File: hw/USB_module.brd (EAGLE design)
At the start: 25 x 45 mm, 39 parts, among them J1 GROVE-4P-2.0-3470130P1, J2 GROVE-4P-2.0-3470130P1, J4 MICRO-USB-5P-340015001, X5 53047-04

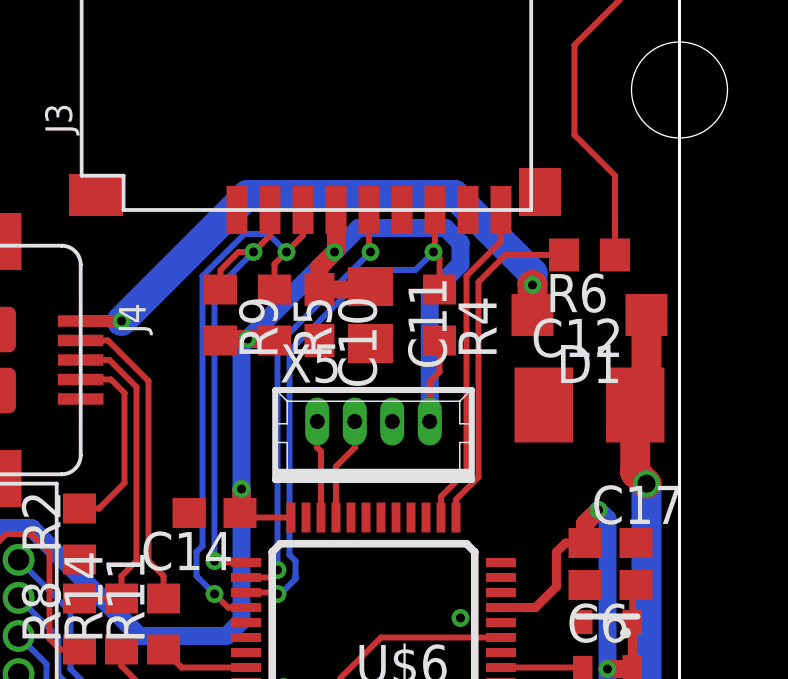
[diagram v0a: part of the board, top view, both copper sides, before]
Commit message: layout completed
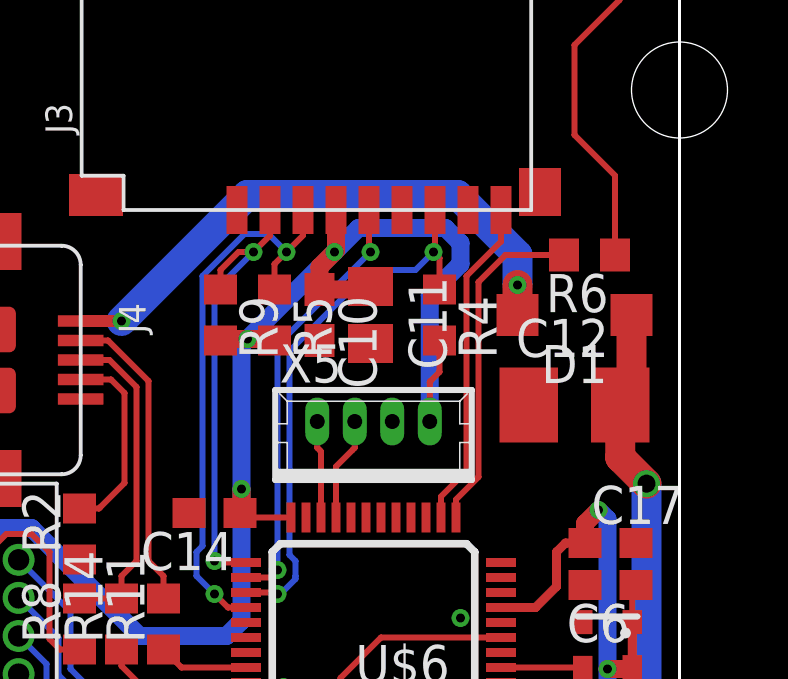
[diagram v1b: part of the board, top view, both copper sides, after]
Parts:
- R4, R5, R9: value 100k -> 47k
- moved C12 0.50 mm to (21.5, 24.5)
- moved D1 0.50 mm to (21.5, 27.5)
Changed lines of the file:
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@@
 <element name="R2" library="rcl" package="R0603" value="100k" x="5" y="20.2" rot="R90"/>
 <element name="R8" library="rcl" package="R0603" value="1k5" x="5" y="17.2" rot="R90"/>
-<element name="D1" library="diode" package="SOD123" value="MBR0520LT" x="22" y="27.5" rot="R180"/>
+<element name="D1" library="diode" package="SOD123" value="MBR0520LT" x="21.5" y="27.5" rot="R180"/>
 <element name="J3" library="OPL-Connector" package="9+4P-SMD-L16.1*W14.5*H1.85MM" value="" x="12.5" y="31" rot="R90"/>
-<element name="R4" library="rcl" package="R0603" value="100k" x="17" y="27.5" rot="R270"/>
-<element name="R5" library="rcl" package="R0603" value="100k" x="11.5" y="27.5" rot="R270"/>
-<element name="R9" library="rcl" package="R0603" value="100k" x="9.7" y="27.5" rot="R270"/>
+<element name="R4" library="rcl" package="R0603" value="47k" x="17" y="27.5" rot="R270"/>
+<element name="R5" library="rcl" package="R0603" value="47k" x="11.5" y="27.5" rot="R270"/>
+<element name="R9" library="rcl" package="R0603" value="47k" x="9.7" y="27.5" rot="R270"/>
 <element name="J4" library="OPL Eagle Library" package="B-SMD-5P" value="MICRO-USB-5P-340015001" x="2.5" y="26" rot="R270"/>
 <element name="C10" library="rcl" package="C0603" value="100n" x="13" y="27.5" rot="R270"/>
 <element name="C11" library="rcl" package="C0805" value="4.7u" x="14.7" y="27.5" rot="R270"/>
-<element name="C12" library="rcl" package="B/3528-21R" value="" x="22" y="24.5"/>
+<element name="C12" library="rcl" package="B/3528-21R" value="" x="21.5" y="24.5"/>
 <element name="LED2" library="led" package="CHIPLED_0805" value="" x="23" y="42.5" rot="R180"/>
 <element name="R6" library="rcl" package="R0603" value="330" x="22" y="29.5" rot="R180"/>
@@
 <contactref element="C12" pad="+"/>
 <via x="23.9" y="21.878" extent="1-16" drill="0.6"/>
-<wire x1="23.9" y1="21.878" x2="23.525" y2="22.253" width="1" layer="1"/>
-<wire x1="23.525" y1="22.253" x2="23.525" y2="24.5" width="1" layer="1"/>
-<wire x1="23.525" y1="24.5" x2="23.9" y2="24.875" width="1" layer="1"/>
-<wire x1="23.9" y1="24.875" x2="23.9" y2="27.5" width="1" layer="1"/>
+<wire x1="23.9" y1="21.878" x2="23.025" y2="22.753" width="1" layer="1"/>
+<wire x1="23.025" y1="22.753" x2="23.025" y2="24.5" width="1" layer="1"/>
+<wire x1="23.025" y1="24.5" x2="23.4" y2="24.875" width="1" layer="1"/>
+<wire x1="23.4" y1="24.875" x2="23.4" y2="27.5" width="1" layer="1"/>
 </signal>
 <signal name="+3V3">
@@
 <wire x1="5.04" y1="27.3" x2="6.4" y2="27.3" width="0.4" layer="1"/>
 <wire x1="6.4" y1="27.3" x2="10.6" y2="31.5" width="1" layer="16"/>
-<wire x1="10.6" y1="31.5" x2="17.5" y2="31.5" width="1" layer="16"/>
-<via x="20.1" y="28.5" extent="1-16" drill="0.3"/>
-<wire x1="20.1" y1="28.5" x2="20.1" y2="27.5" width="1" layer="1"/>
-<wire x1="17.5" y1="31.5" x2="20.1" y2="28.9" width="1" layer="16"/>
-<wire x1="20.1" y1="28.9" x2="20.1" y2="28.5" width="1" layer="16"/>
+<wire x1="10.6" y1="31.5" x2="17.6" y2="31.5" width="1" layer="16"/>
+<via x="19.6" y="28.5" extent="1-16" drill="0.3"/>
+<wire x1="19.6" y1="28.5" x2="19.6" y2="27.5" width="1" layer="1"/>
+<wire x1="17.6" y1="31.5" x2="19.6" y2="29.5" width="1" layer="16"/>
+<wire x1="19.6" y1="29.5" x2="19.6" y2="28.5" width="1" layer="16"/>
 </signal>
 <signal name="USB_N">
